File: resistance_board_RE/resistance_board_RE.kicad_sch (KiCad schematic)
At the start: 38 parts, among them J1 Red Wire, J2 Blrown Wire, J3 Yellow Wire, J4 Black Wire, Q1 FZT658, Q2 SOT_23 Device "GM X", Q3 04N80C3, Q4 FZT758, Q5 TIP32CG Heatsunk, Q6 Q_PMOS_GDS, U1 PVI5080N, U2 LTC1052CSW-PBF, U3 PVI5080N, U4 LTC1150

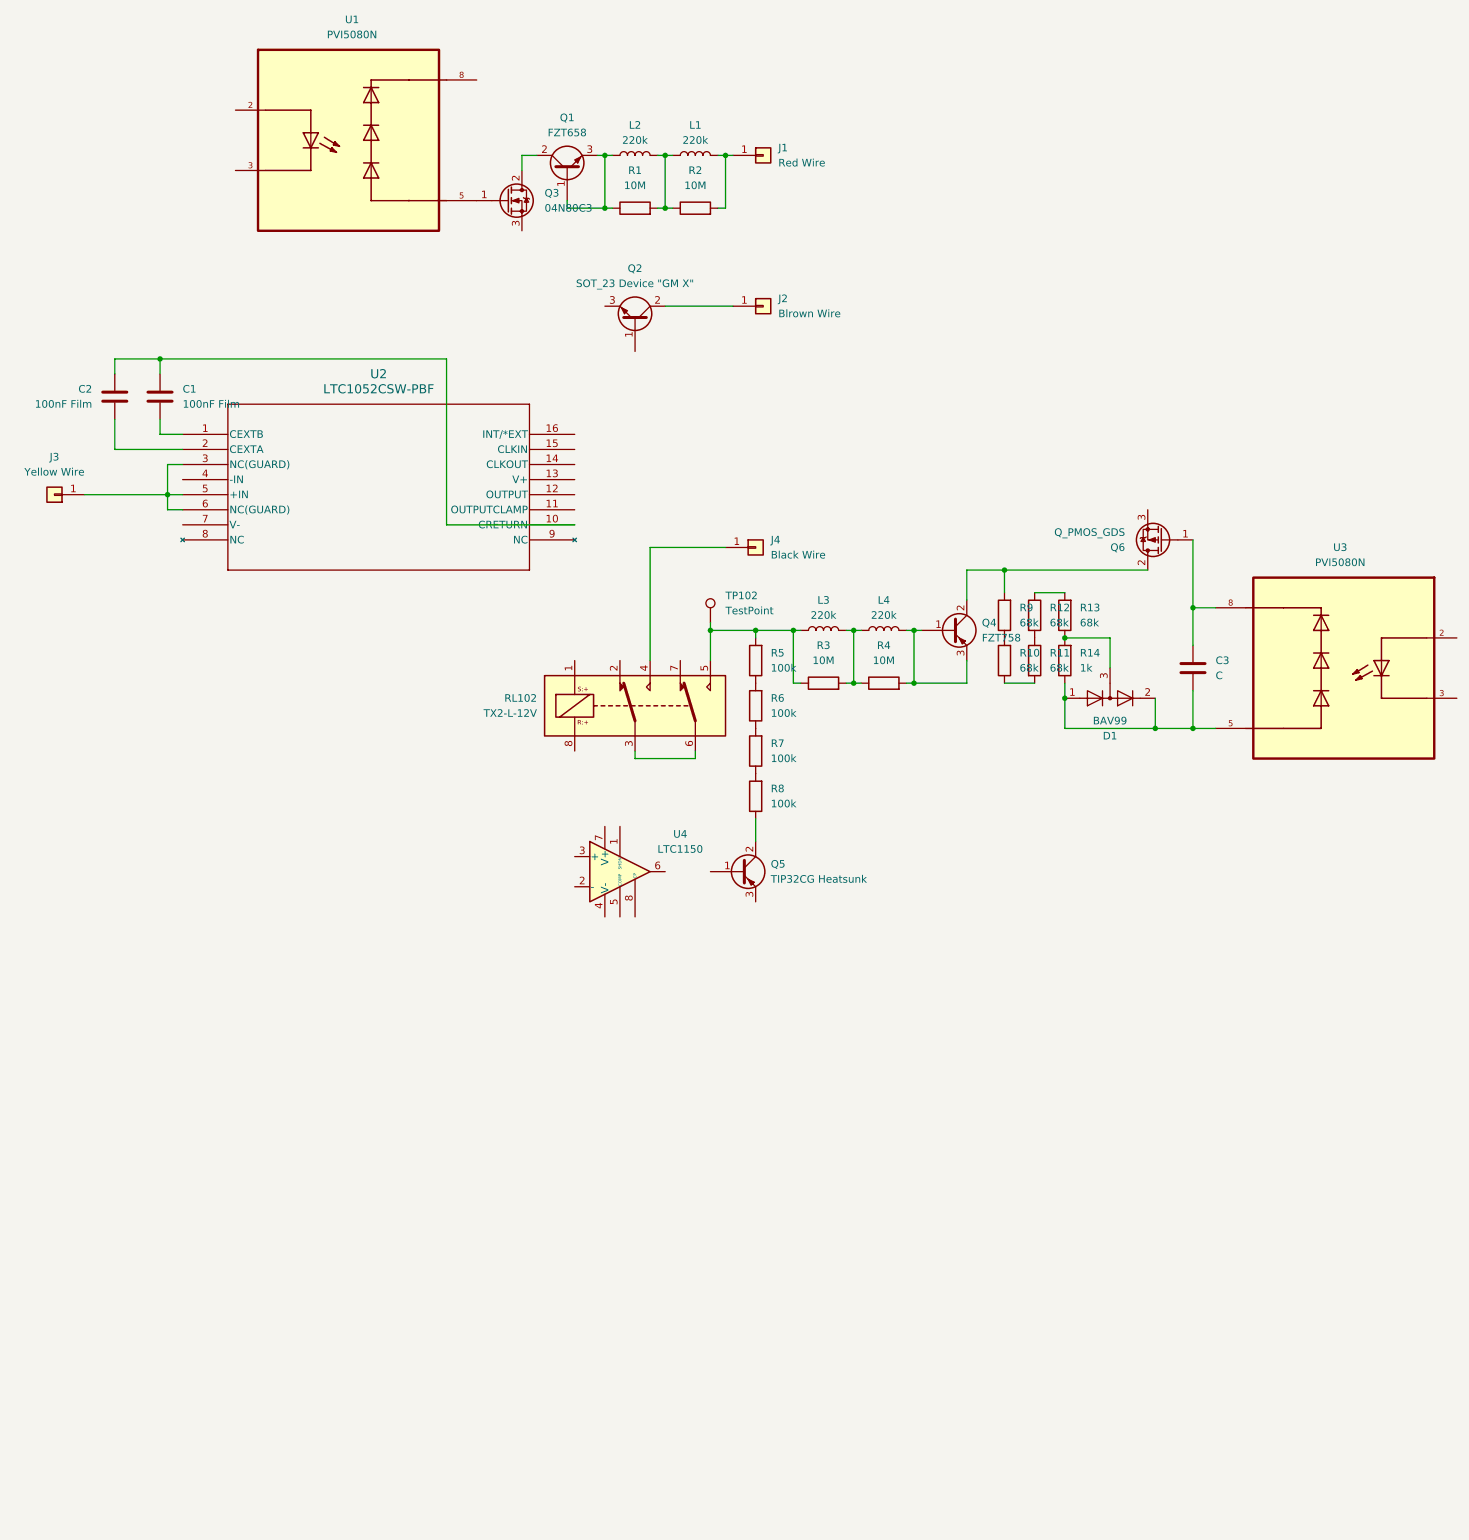
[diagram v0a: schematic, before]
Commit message: asdf
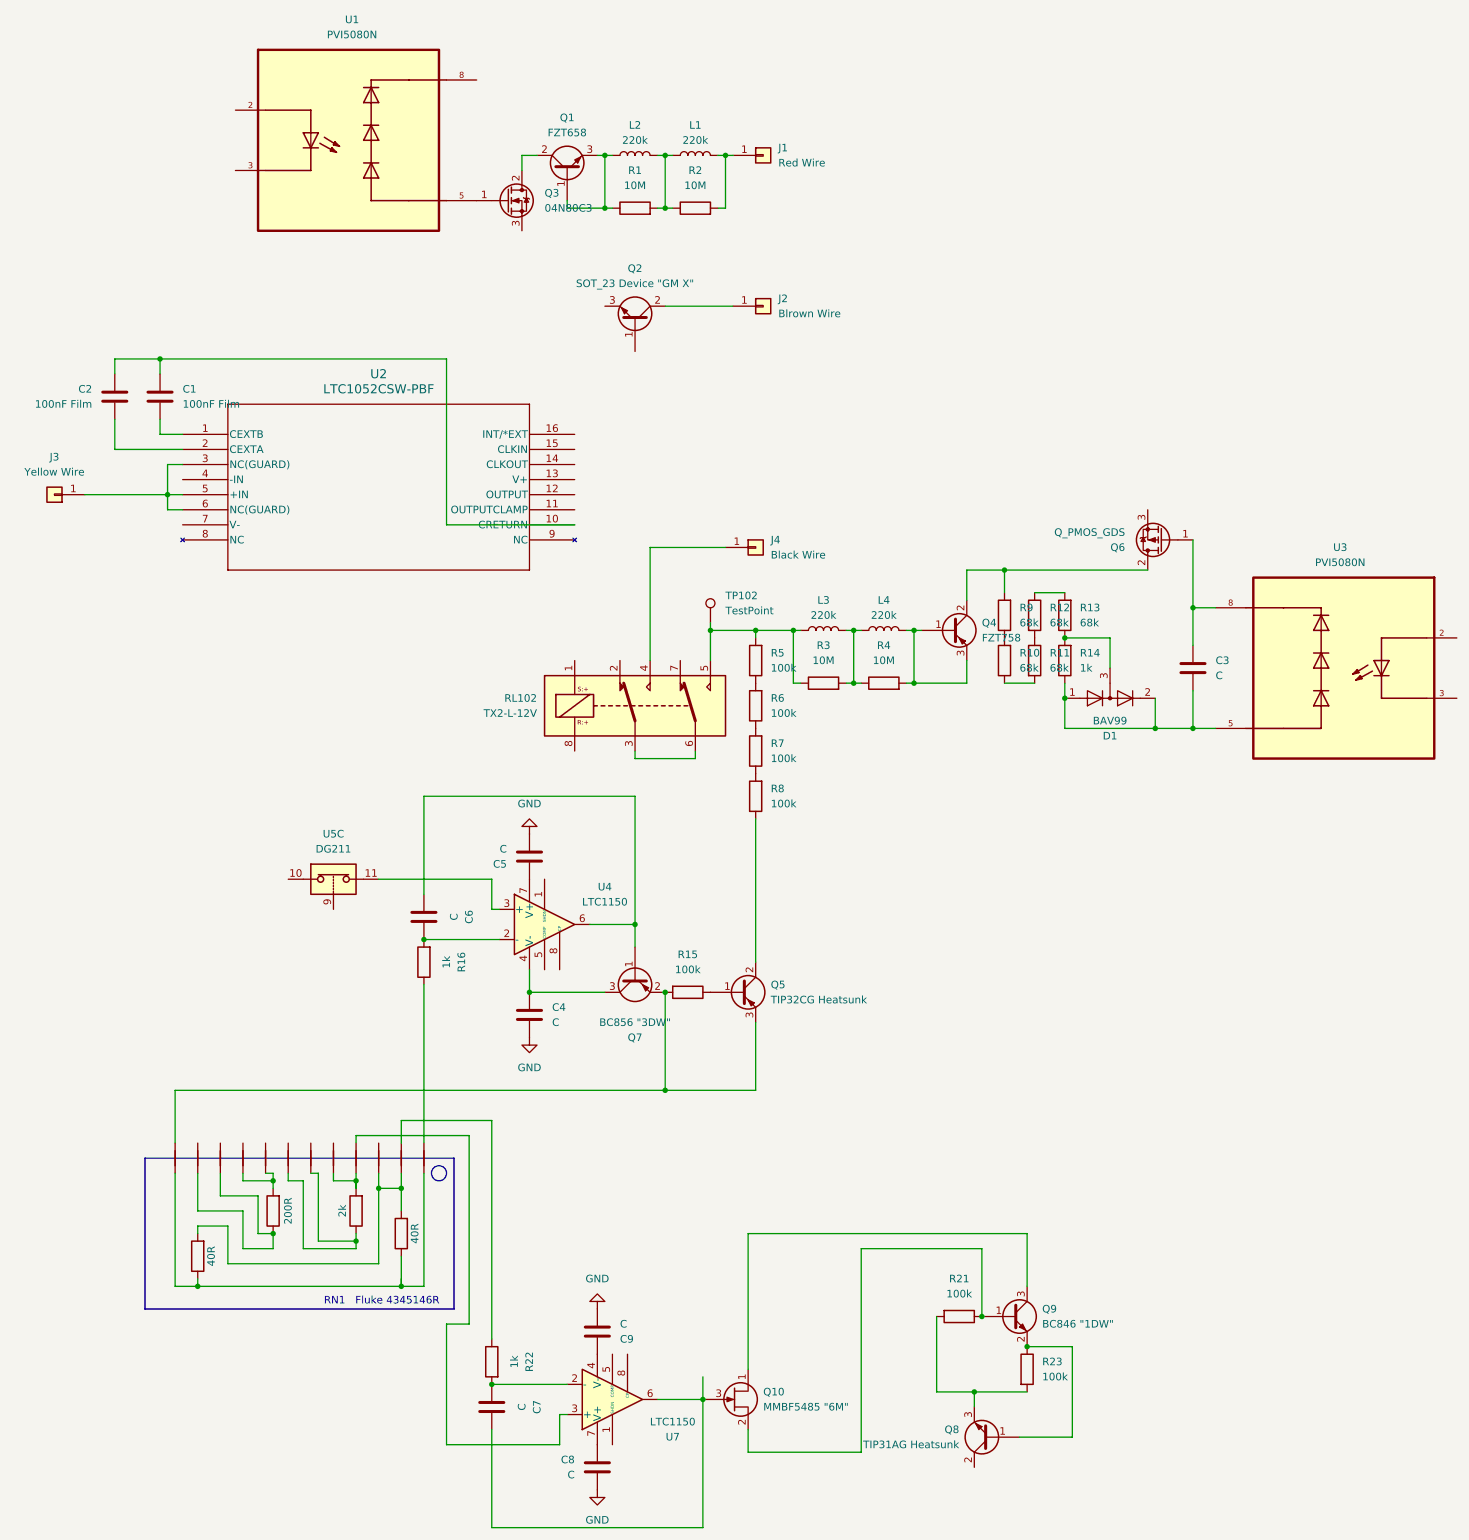
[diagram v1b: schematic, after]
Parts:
- added C4, C5, C6, C7, C8, C9: C, symbol Device:C
- added NT1, NT10, NT11, NT12, NT2, NT3, NT4, NT5, NT6, NT7, NT8, NT9: NetTie_2, symbol Device:NetTie_2
- added Q10: MMBF5485 "6M", symbol Device:Q_NJFET_DSG
- added Q7: BC856 "3DW", symbol Device:Q_PNP_BEC
- added Q8: TIP31AG Heatsunk, symbol Device:Q_NPN_BCE
- added Q9: BC846 "1DW", symbol Device:Q_NPN_BEC
- added R15, R21, R23: 100k, symbol Device:R
- added R16, R22: 1k, symbol Device:R
- added R17, R20: 40R, symbol Device:R
- added R18: 200R, symbol Device:R
- added R19: 2k, symbol Device:R
- added U5: DG211, Package_SO:SOIC-16_3.9x9.9mm_P1.27mm, symbol Analog_Switch:DG411xY
- added U7: LTC1150, symbol Amplifier_Operational:LTC1152
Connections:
- net at U4.2 (-): now also C6.2, R16.2
- net at U4.3 (+): now also U5.11
- net at U4.4 (V-): now also C4.1, Q7.3 (C)
- net at U4.6: now also C6.1, Q7.1 (B)
- net at U4.7 (V+): now also C5.1
- net at Q5.1 (B): now also R15.1
- net at Q5.3 (E): now also NT4.2, Q7.2 (E), R15.2
- new net: NT10.1, NT9.1, R18.1
- new net: NT11.1, NT12.1, R18.2
- new net: C9.1, U7.4 (V-)
- new net: Q8.1 (B), Q9.2 (E), R23.1
- new net: Q8.3 (E), R21.2, R23.2
- new net: C7.1, Q10.3 (G), U7.6
- new net: C7.2, R22.2, U7.2 (-)
- new net: NT5.1, NT8.1, R19.1
- new net: NT6.1, NT7.1, R19.2
- new net: NT2.1, NT3.1, R17.2, R20.2
- new net: NT2.2, R22.1
- new net: NT1.1, NT4.1, R17.1, R20.1
- new net: Q10.1 (D), Q9.3 (C)
- new net: Q10.2 (S), Q9.1 (B), R21.1
- new net: NT7.2, U7.3 (+)
- new net: C8.1, U7.7 (V+)
- new net: NT1.2, R16.1
- new net GND: C4.2, C5.2, C8.2, C9.2
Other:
- note added: "RN1 Fluke 4345146R"
- moved on the sheet: Q5, U4
